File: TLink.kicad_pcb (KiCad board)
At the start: 2 copper layers, 34.5 x 34 mm, 5 parts, among them J1 Conn_02x10_Odd_Even, J2 Conn_02x05_Odd_Even, J3 Conn_02x05_Odd_Even, J4 Conn_01x03, J5 Conn_01x02

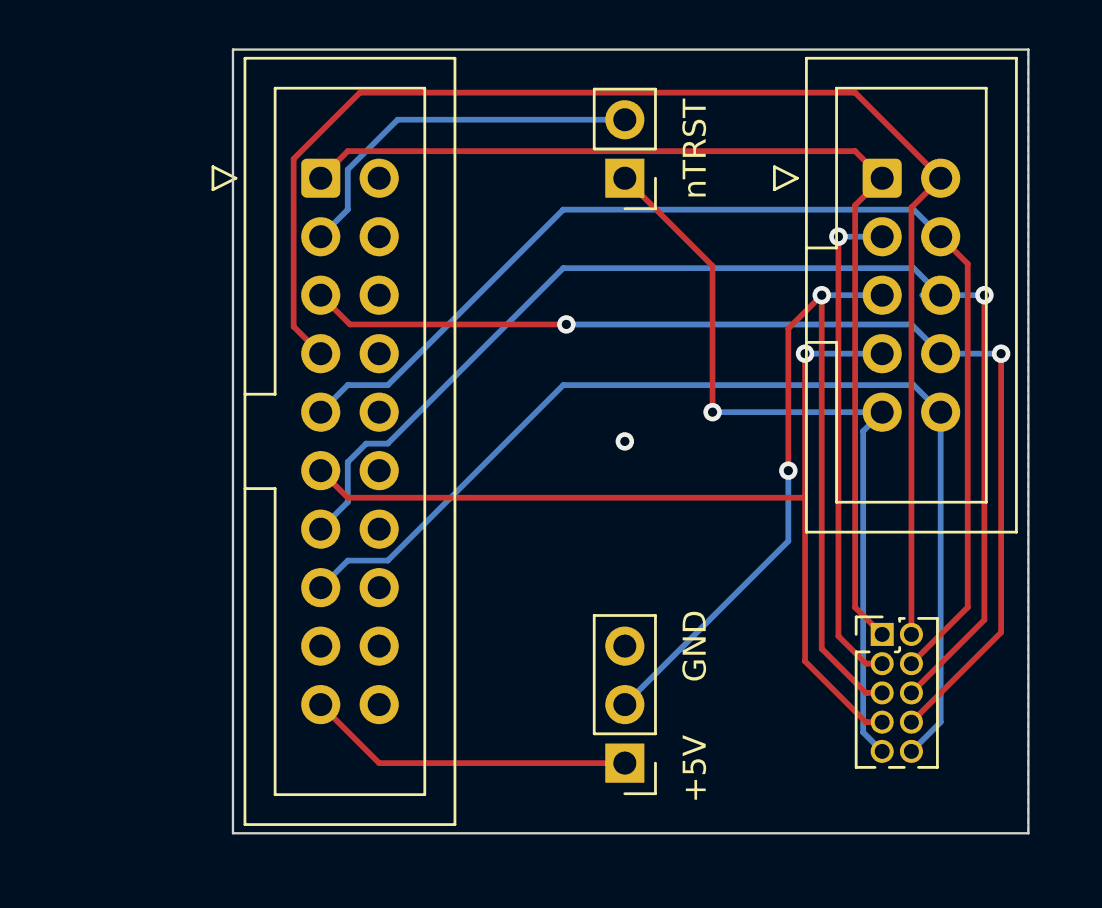
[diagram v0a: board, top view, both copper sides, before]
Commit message: Make the board more handy
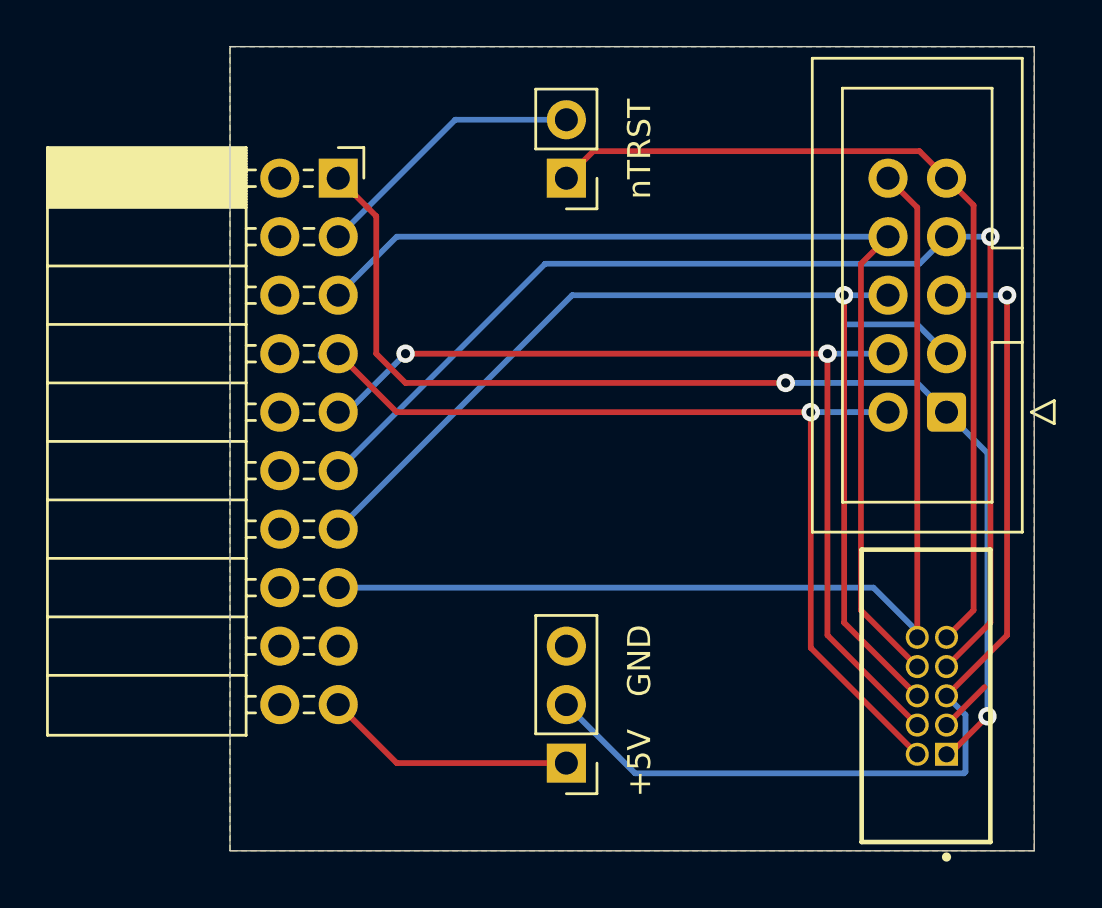
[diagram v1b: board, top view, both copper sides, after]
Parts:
- J1: footprint Connector_IDC:IDC-Header_2x10_P2.54mm_Vertical -> Connector_PinSocket_2.54mm:PinSocket_2x10_P2.54mm_Horizontal
- J3: footprint Connector_PinHeader_1.27mm:PinHeader_2x05_P1.27mm_Vertical -> SHF-105-01-L-D-TH:SHF-105-01-L-D-TH
- moved J2 10.5 mm to (88.9, 55.9), turned to 180 degrees
- moved J3 5.91 mm to (88.9, 70.7), turned to 90 degrees
- moved J4 2.54 mm to (72.4, 71.1)
- moved J5 2.54 mm to (72.4, 45.7)
- moved J1 0.76 mm to (62.5, 45.7)
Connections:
- J1 pad 10: (no net) -> GND
- J1 pad 12: (no net) -> GND
- J1 pad 14: (no net) -> Net-(J1-Pad14)
- J1 pad 16: (no net) -> Net-(J1-Pad16)
- J1 pad 17: (no net) -> Net-(J1-Pad17)
- J1 pad 18: (no net) -> Net-(J1-Pad18)
- J1 pad 2: (no net) -> Net-(J1-Pad2)
- J1 pad 20: (no net) -> Net-(J1-Pad20)
- J1 pad 6: (no net) -> GND
- J1 pad 8: (no net) -> GND
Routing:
- net Net-(J1-Pad7): track 60.1 -> 42.2 mm, vias 0 -> 1
- net GND: track 21.6 -> 7.31 mm, vias 2 -> 0
- net Net-(J1-Pad11): track 42.7 -> 52.0 mm
- net Net-(J1-Pad9): track 51.1 -> 42.9 mm, vias 0 -> 2
- net Net-(J1-Pad13): track 54.4 -> 46.8 mm
- net Net-(J1-Pad1): track 46.1 -> 51.0 mm, vias 0 -> 2
- net Net-(J1-Pad3): track 16.3 -> 12.0 mm
- net Net-(J2-Pad9): track 34.5 -> 38.4 mm, vias 1 -> 0
- net +5V: track 14.3 -> 11.0 mm
- net Net-(J1-Pad5): track 48.2 -> 45.1 mm, vias 2 -> 0
- net Net-(J2-Pad5): track 42.7 -> 44.0 mm, vias 2 -> 1
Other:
- board size 34.5 x 34 mm -> 34.9 x 34.9 mm
